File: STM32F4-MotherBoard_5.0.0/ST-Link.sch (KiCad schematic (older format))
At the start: 5 parts

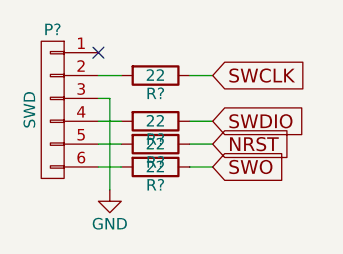
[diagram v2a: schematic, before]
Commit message: 回路図終わり
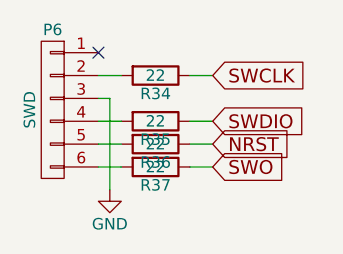
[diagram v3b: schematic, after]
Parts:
- gave numbers to parts that had none: 5
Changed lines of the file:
@@
 $Descr A4 11693 8268
 encoding utf-8
-Sheet 8 11
+Sheet 8 12
 Title ""
 Date ""
@@
 $EndDescr
 $Comp
-L CONN_01X06 P?
+L CONN_01X06 P6
 U 1 1 589F4C21
 P 5650 3050
-F 0 "P?" H 5650 3400 50  0000 C CNN
+F 0 "P6" H 5650 3400 50  0000 C CNN
 F 1 "SWD" V 5750 3050 50  0000 C CNN
 F 2 "" H 5650 3050 50  0000 C CNN
@@
 $EndComp
 $Comp
-L R R?
+L R R34
 U 1 1 589F4C7C
 P 6100 2900
-F 0 "R?" V 6180 2900 50  0000 C CNN
+F 0 "R34" V 6180 2900 50  0000 C CNN
 F 1 "22" V 6100 2900 50  0000 C CNN
 F 2 "" V 6030 2900 50  0000 C CNN
@@
 $EndComp
 $Comp
-L R R?
+L R R35
 U 1 1 589F4CC4
 P 6100 3100
-F 0 "R?" V 6180 3100 50  0000 C CNN
+F 0 "R35" V 6180 3100 50  0000 C CNN
 F 1 "22" V 6100 3100 50  0000 C CNN
 F 2 "" V 6030 3100 50  0000 C CNN
@@
 $EndComp
 $Comp
-L R R?
+L R R36
 U 1 1 589F4CE0
 P 6100 3200
-F 0 "R?" V 6180 3200 50  0000 C CNN
+F 0 "R36" V 6180 3200 50  0000 C CNN
 F 1 "22" V 6100 3200 50  0000 C CNN
 F 2 "" V 6030 3200 50  0000 C CNN
@@
 $EndComp
 $Comp
-L R R?
+L R R37
 U 1 1 589F4D03
 P 6100 3300
-F 0 "R?" V 6180 3300 50  0000 C CNN
+F 0 "R37" V 6180 3300 50  0000 C CNN
 F 1 "22" V 6100 3300 50  0000 C CNN
 F 2 "" V 6030 3300 50  0000 C CNN
@@
 	5900 3000 5900 3400
 $Comp
-L GND #PWR?
+L GND #PWR063
 U 1 1 589F4E4F
 P 5900 3400
-F 0 "#PWR?" H 5900 3150 50  0001 C CNN
+F 0 "#PWR063" H 5900 3150 50  0001 C CNN
 F 1 "GND" H 5900 3250 50  0000 C CNN
 F 2 "" H 5900 3400 50  0000 C CNN

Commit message: 部品名変更
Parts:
- P6: footprint (none) -> mylib:PinHeader-6
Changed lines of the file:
@@
 EESchema Schematic File Version 2
+LIBS:STM32F4-MotherBoard_5.0.0-rescue
 LIBS:power
 LIBS:device
@@
 F 0 "P6" H 5650 3400 50  0000 C CNN
 F 1 "SWD" V 5750 3050 50  0000 C CNN
-F 2 "" H 5650 3050 50  0000 C CNN
+F 2 "mylib:PinHeader-6" H 5650 3050 50  0001 C CNN
 F 3 "" H 5650 3050 50  0000 C CNN
 	1    5650 3050
@@
 F 0 "R34" V 6180 2900 50  0000 C CNN
 F 1 "22" V 6100 2900 50  0000 C CNN
-F 2 "" V 6030 2900 50  0000 C CNN
+F 2 "" V 6030 2900 50  0001 C CNN
 F 3 "" H 6100 2900 50  0000 C CNN
 	1    6100 2900
@@
 F 0 "R35" V 6180 3100 50  0000 C CNN
 F 1 "22" V 6100 3100 50  0000 C CNN
-F 2 "" V 6030 3100 50  0000 C CNN
+F 2 "" V 6030 3100 50  0001 C CNN
 F 3 "" H 6100 3100 50  0000 C CNN
 	1    6100 3100
@@
 F 0 "R36" V 6180 3200 50  0000 C CNN
 F 1 "22" V 6100 3200 50  0000 C CNN
-F 2 "" V 6030 3200 50  0000 C CNN
+F 2 "" V 6030 3200 50  0001 C CNN
 F 3 "" H 6100 3200 50  0000 C CNN
 	1    6100 3200
@@
 F 0 "R37" V 6180 3300 50  0000 C CNN
 F 1 "22" V 6100 3300 50  0000 C CNN
-F 2 "" V 6030 3300 50  0000 C CNN
+F 2 "" V 6030 3300 50  0001 C CNN
 F 3 "" H 6100 3300 50  0000 C CNN
 	1    6100 3300
@@
 	5900 3000 5900 3400
 $Comp
-L GND #PWR063
+L GND #PWR065
 U 1 1 589F4E4F
 P 5900 3400
-F 0 "#PWR063" H 5900 3150 50  0001 C CNN
+F 0 "#PWR065" H 5900 3150 50  0001 C CNN
 F 1 "GND" H 5900 3250 50  0000 C CNN
 F 2 "" H 5900 3400 50  0000 C CNN

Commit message: 関連付けできたの
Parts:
- R34, R35, R36, R37: footprint (none) -> robocon_pcb:SM0603_EXP0.5mm
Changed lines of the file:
@@
 F 0 "R34" V 6180 2900 50  0000 C CNN
 F 1 "22" V 6100 2900 50  0000 C CNN
-F 2 "" V 6030 2900 50  0001 C CNN
+F 2 "robocon_pcb:SM0603_EXP0.5mm" V 6030 2900 50  0001 C CNN
 F 3 "" H 6100 2900 50  0000 C CNN
 	1    6100 2900
@@
 F 0 "R35" V 6180 3100 50  0000 C CNN
 F 1 "22" V 6100 3100 50  0000 C CNN
-F 2 "" V 6030 3100 50  0001 C CNN
+F 2 "robocon_pcb:SM0603_EXP0.5mm" V 6030 3100 50  0001 C CNN
 F 3 "" H 6100 3100 50  0000 C CNN
 	1    6100 3100
@@
 F 0 "R36" V 6180 3200 50  0000 C CNN
 F 1 "22" V 6100 3200 50  0000 C CNN
-F 2 "" V 6030 3200 50  0001 C CNN
+F 2 "robocon_pcb:SM0603_EXP0.5mm" V 6030 3200 50  0001 C CNN
 F 3 "" H 6100 3200 50  0000 C CNN
 	1    6100 3200
@@
 F 0 "R37" V 6180 3300 50  0000 C CNN
 F 1 "22" V 6100 3300 50  0000 C CNN
-F 2 "" V 6030 3300 50  0001 C CNN
+F 2 "robocon_pcb:SM0603_EXP0.5mm" V 6030 3300 50  0001 C CNN
 F 3 "" H 6100 3300 50  0000 C CNN
 	1    6100 3300
@@
 	5900 3000 5900 3400
 $Comp
-L GND #PWR065
+L GND #PWR069
 U 1 1 589F4E4F
 P 5900 3400
-F 0 "#PWR065" H 5900 3150 50  0001 C CNN
+F 0 "#PWR069" H 5900 3150 50  0001 C CNN
 F 1 "GND" H 5900 3250 50  0000 C CNN
 F 2 "" H 5900 3400 50  0000 C CNN
